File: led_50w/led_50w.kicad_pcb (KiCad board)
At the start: 2 copper layers, 120 x 80 mm, 49 parts

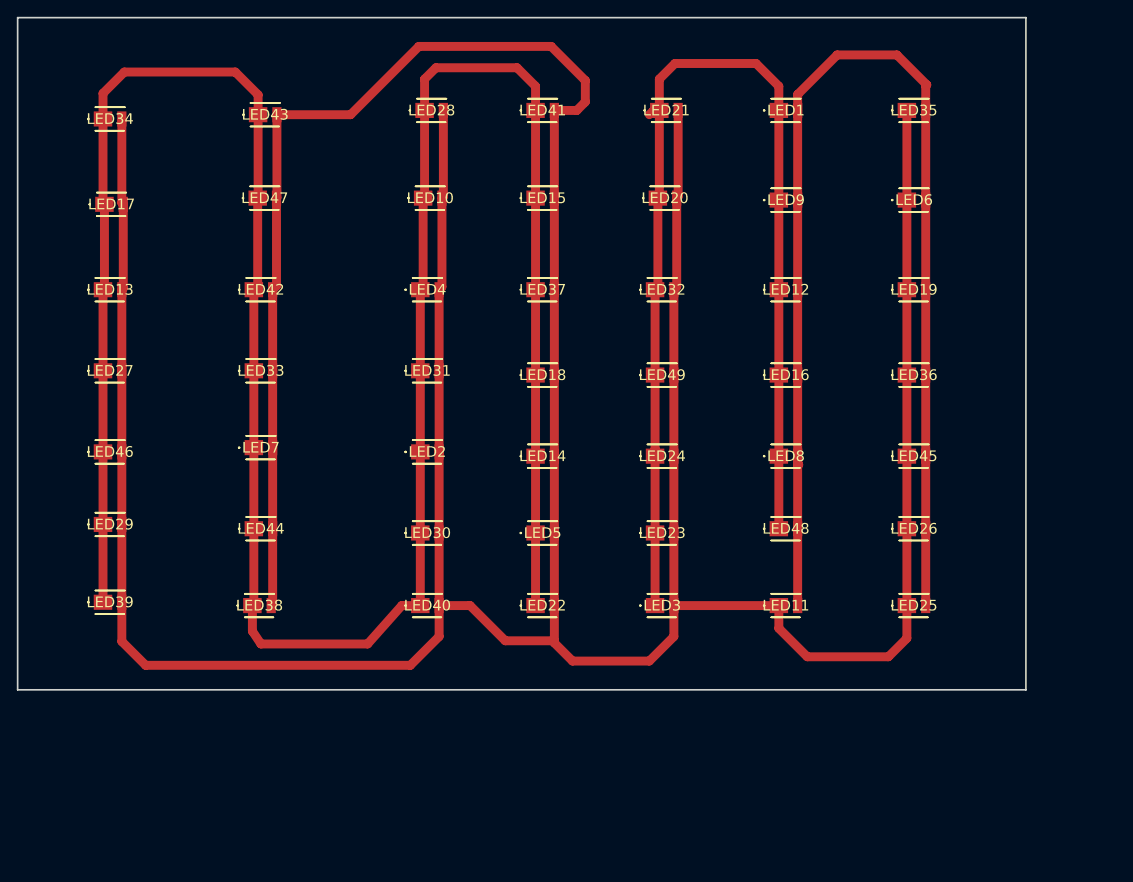
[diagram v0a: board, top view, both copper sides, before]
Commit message: rev 2 eeschema&layout
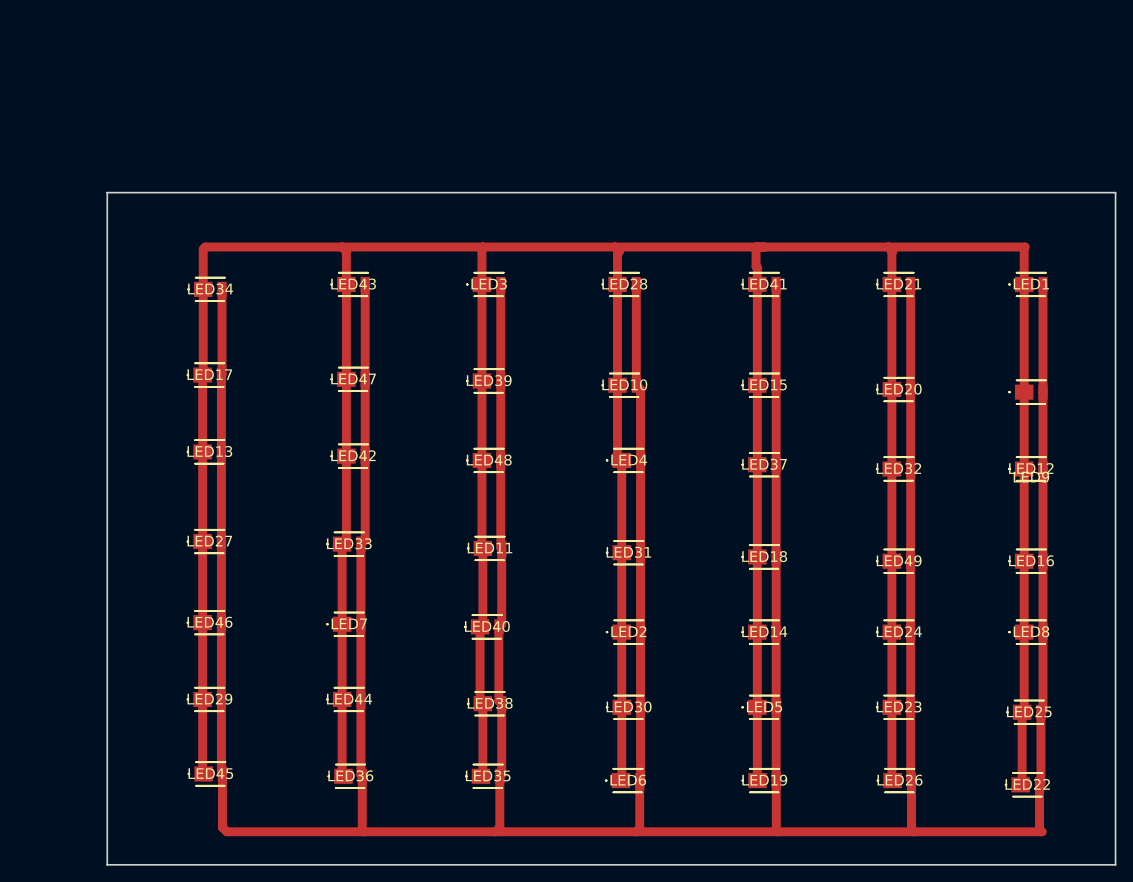
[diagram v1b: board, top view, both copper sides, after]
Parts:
- moved LED35 94.1 mm to (111.0, 131.6)
- moved LED45 91.8 mm to (78.0, 131.3)
- moved LED36 82.3 mm to (94.7, 131.6)
- moved LED6 77.0 mm to (127.7, 132.1)
- moved LED22 61.6 mm to (175.3, 132.6)
- moved LED19 61.1 mm to (143.9, 132.1)
- moved LED39 52.2 mm to (111.1, 84.5)
- moved LED3 43.4 mm to (111.1, 73.0)
- moved LED9 37.1 mm to (175.7, 85.9)
- moved LED16 36.7 mm to (175.7, 106.0)
- moved LED48 36.3 mm to (111.1, 94.0)
- moved LED12 36.2 mm to (175.7, 95.0)
- moved LED20 36.0 mm to (159.9, 85.5)
- moved LED8 35.9 mm to (175.7, 114.4)
- moved LED11 35.9 mm to (111.3, 104.5)
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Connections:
- LED11 pad 1: +24V -> GND
- LED19 pad 1: +24V -> GND
- LED25 pad 1: +24V -> GND
- LED26 pad 1: +24V -> GND
- LED35 pad 1: +24V -> GND
- LED36 pad 1: +24V -> GND
- LED45 pad 1: +24V -> GND
- LED6 pad 1: +24V -> GND
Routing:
- net +24V: track 667.9 -> 554.6 mm
- net GND: track 441.6 -> 542.9 mm
